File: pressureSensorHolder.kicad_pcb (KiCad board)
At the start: 2 copper layers, 29 x 18 mm, 2 parts, among them J1 Conn_01x04, U1 SDP8xx-ANALOG

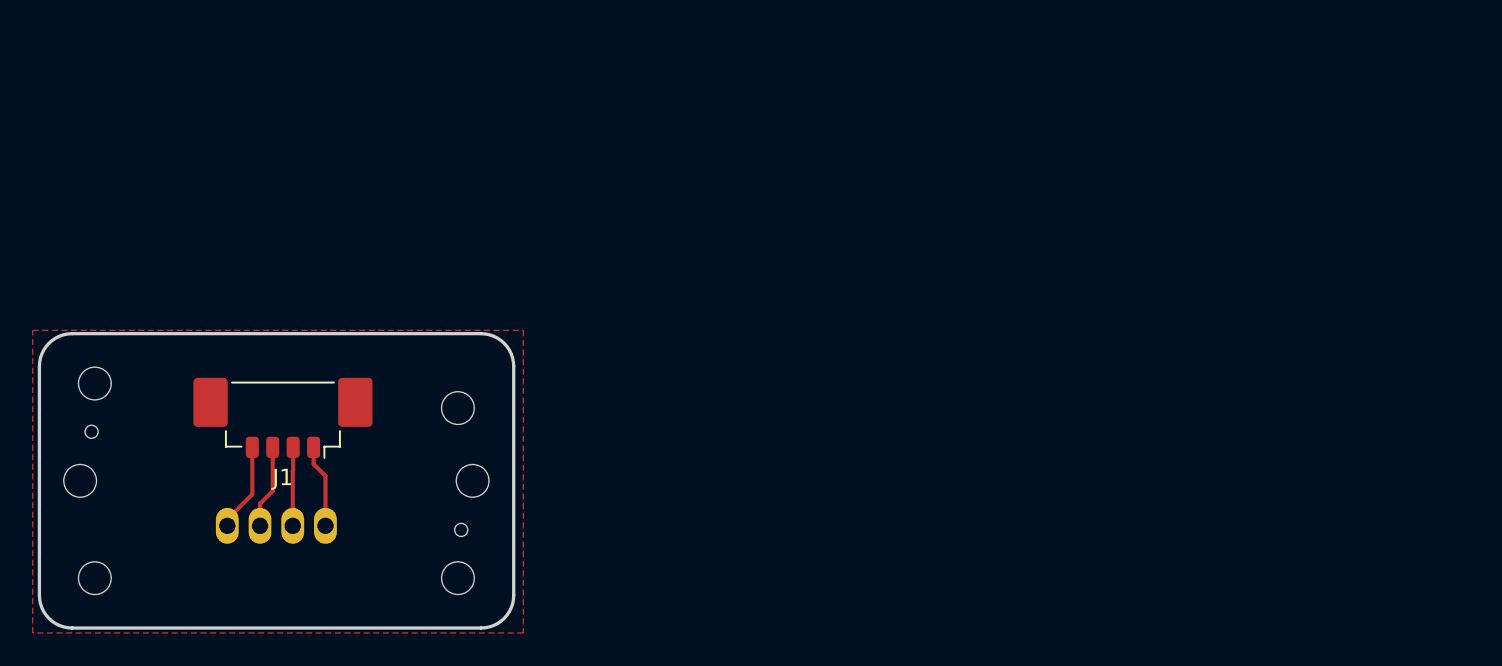
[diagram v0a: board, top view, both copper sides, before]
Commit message: New JST(PH) connection and mounting holes
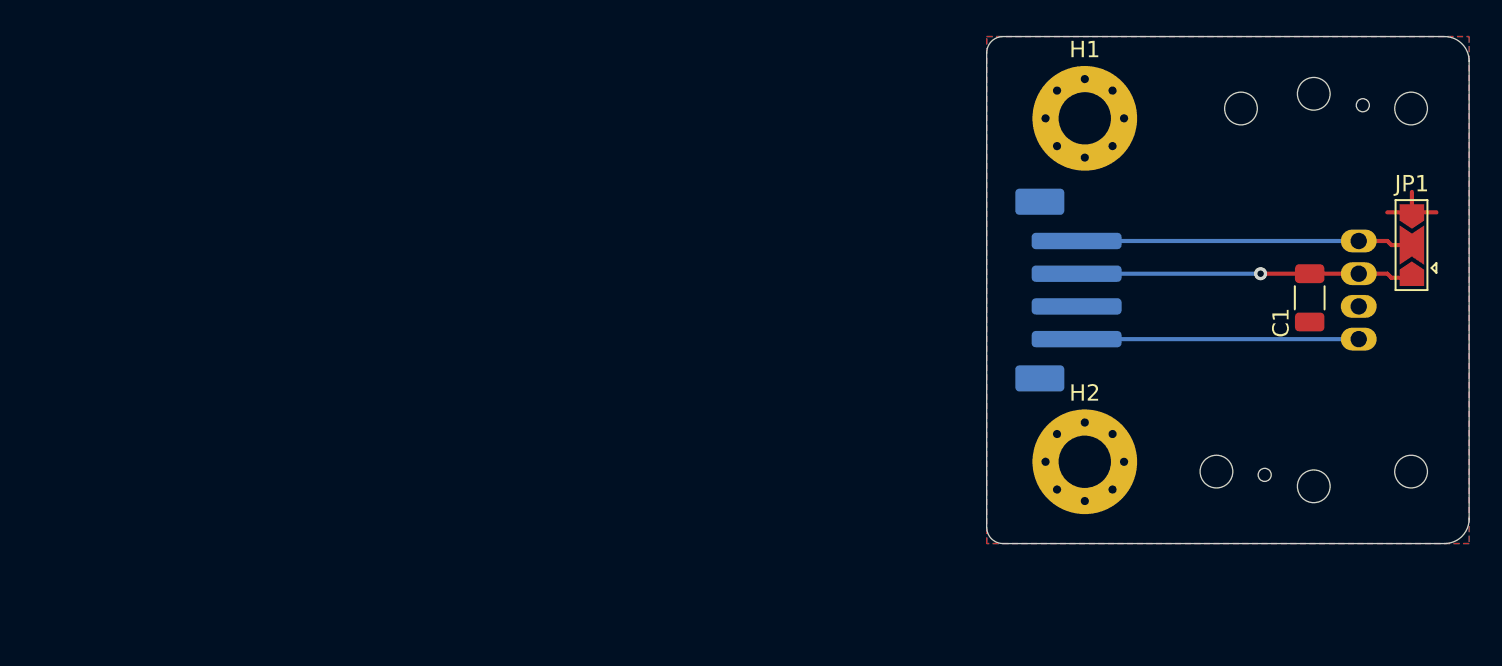
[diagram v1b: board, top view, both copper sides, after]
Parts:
- added C1: C, Capacitor_SMD:C_1206_3216Metric, F.Cu at (148.7, 84.1)
- added H1: MountingHole, MountingHole:MountingHole_3.2mm_M3_Pad_Via, F.Cu at (134.9, 73.2)
- added H2: MountingHole, MountingHole:MountingHole_3.2mm_M3_Pad_Via, F.Cu at (134.9, 94.2)
- added JP1: SolderJumper_3_Open, Jumper:SolderJumper-3_P2.0mm_Open_TrianglePad1.0x1.5mm, F.Cu at (154.9, 80.9)
- J1: footprint Connector_Molex:Molex_PicoBlade_53398-0471_1x04-1MP_P1.25mm_Vertical -> Connector_JST:JST_PH_B4B-PH-SM4-TB_1x04-1MP_P2.00mm_Vertical; moved to B.Cu
- moved U1 64.5 mm to (148.9, 83.7), turned to 270 degrees
- moved J1 48.8 mm to (133.9, 83.7), turned to 270 degrees
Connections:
- net /GND renamed GND
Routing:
- net /Vdd: track 4.81 -> 20.6 mm, vias 0 -> 1
- net /OCS_SCL: track 5.10 -> 20.6 mm
- net /AOut_SDA: track 5.43 -> 17.2 mm
- net GND: track 5.12 -> 4.25 mm
- added copper zone on B.Cu, net GND
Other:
- board size 29 x 18 mm -> 29.5 x 31 mm
- net class Default: clearance 0.2 -> 0.254; trace_width 0.25 -> 0.254
- rule trace_clearance: 0.2 -> 0.254
- rule trace_min: 0.2 -> 0.1
